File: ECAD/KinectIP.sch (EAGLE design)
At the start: 4 parts, among them P5+ 2PIN-FEMALE-HEADER

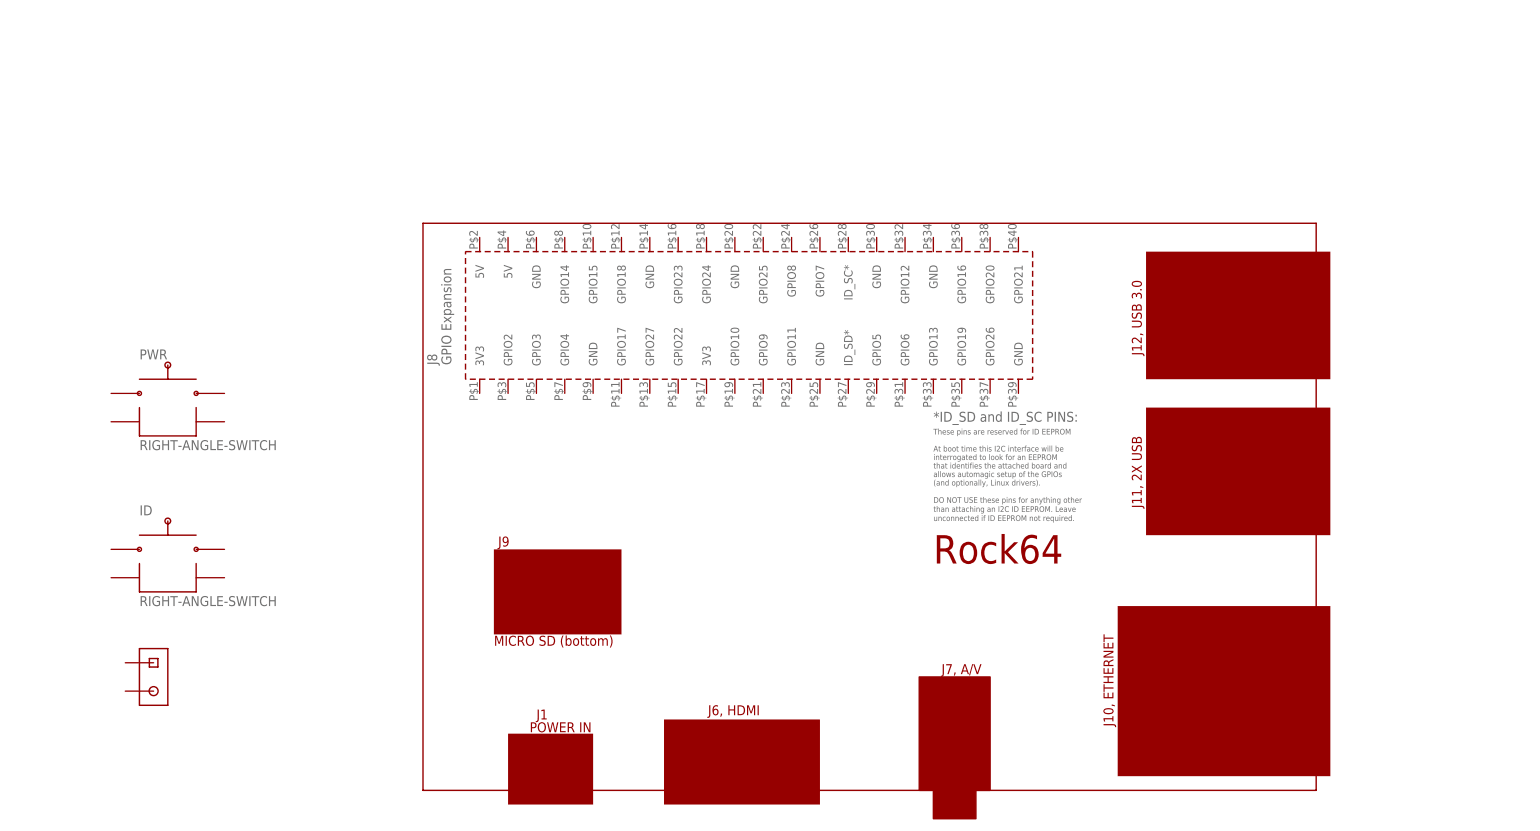
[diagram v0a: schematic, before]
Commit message: add lbr
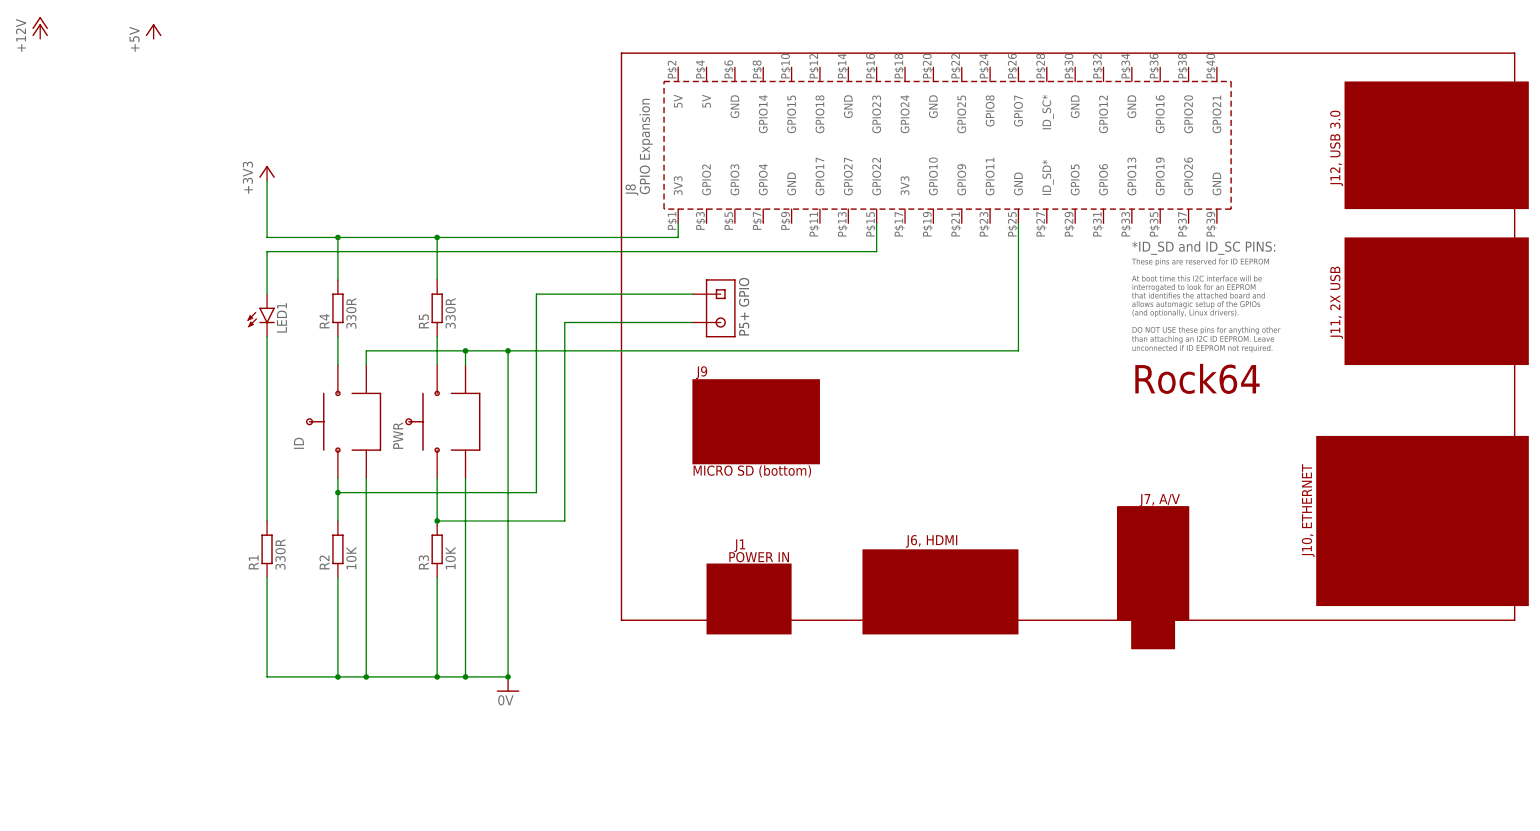
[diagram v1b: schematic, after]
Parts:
- added LED1: (no value), led:LED3MM
- added R1, R4, R5: 330R, rcl:R-EU_R0805
- added R2, R3: 10K, rcl:R-EU_R0805
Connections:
- new net +3V3: PCB2.3V3@1, R4.2, R5.2
- new net 0V: ID.MNT$1, ID.MNT$2, PCB2.GND@25, PWR.MNT$1, PWR.MNT$2, R1.1, R2.1, R3.1
- new net N$1: LED1.A, PCB2.GPIO22
- new net N$2: LED1.C, R1.2
- new net N$3: ID.SW$2, R4.1
- new net N$4: PWR.SW$2, R5.1
- new net N$5: ID.SW$1, P5+.P$1, R2.2
- new net N$6: P5+.P$2, PWR.SW$1, R3.2
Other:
- note added: "P5+ GPIO"
- moved on the sheet: ID, PWR
